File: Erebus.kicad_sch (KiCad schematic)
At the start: 1 part, among them U1 STM32F303CBTx

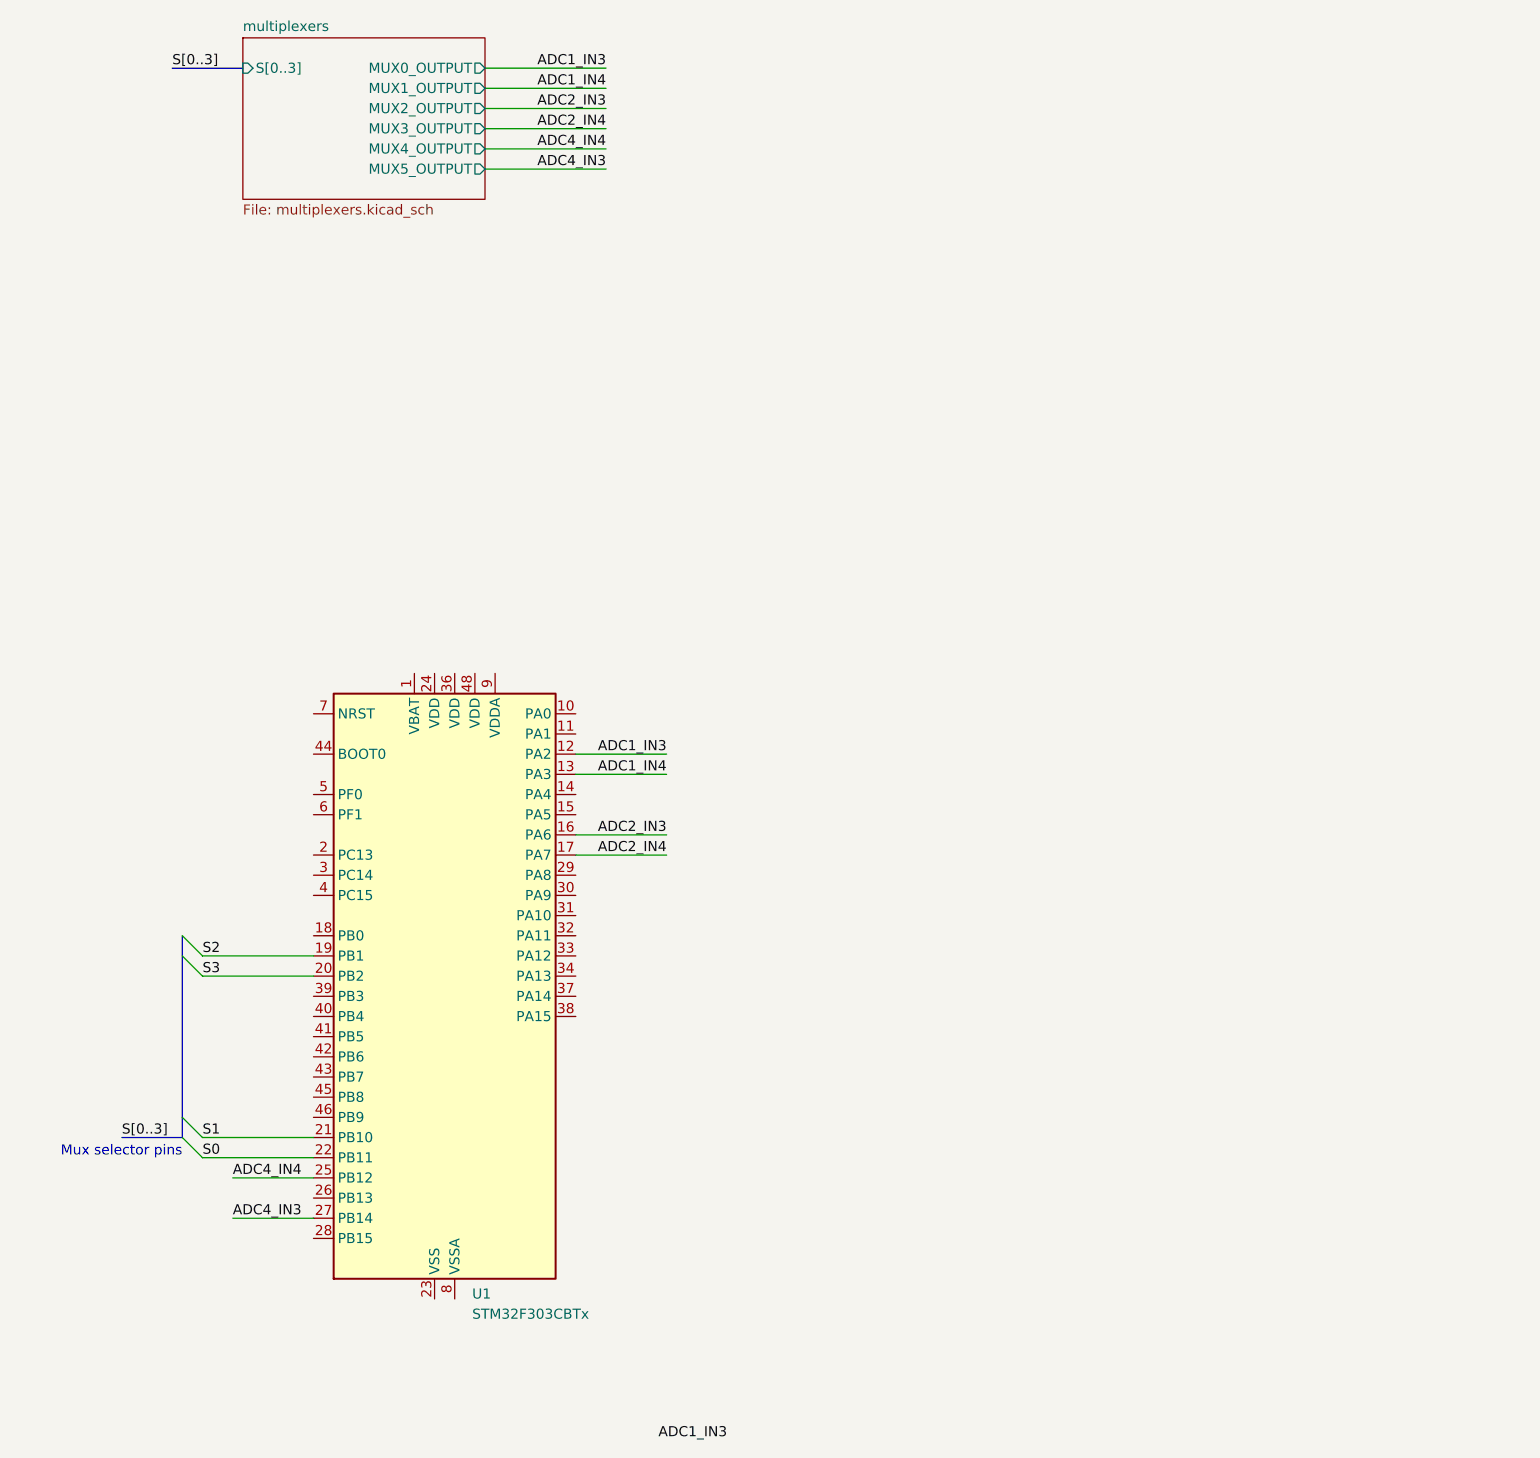
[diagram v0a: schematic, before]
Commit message: Setup Base Layout
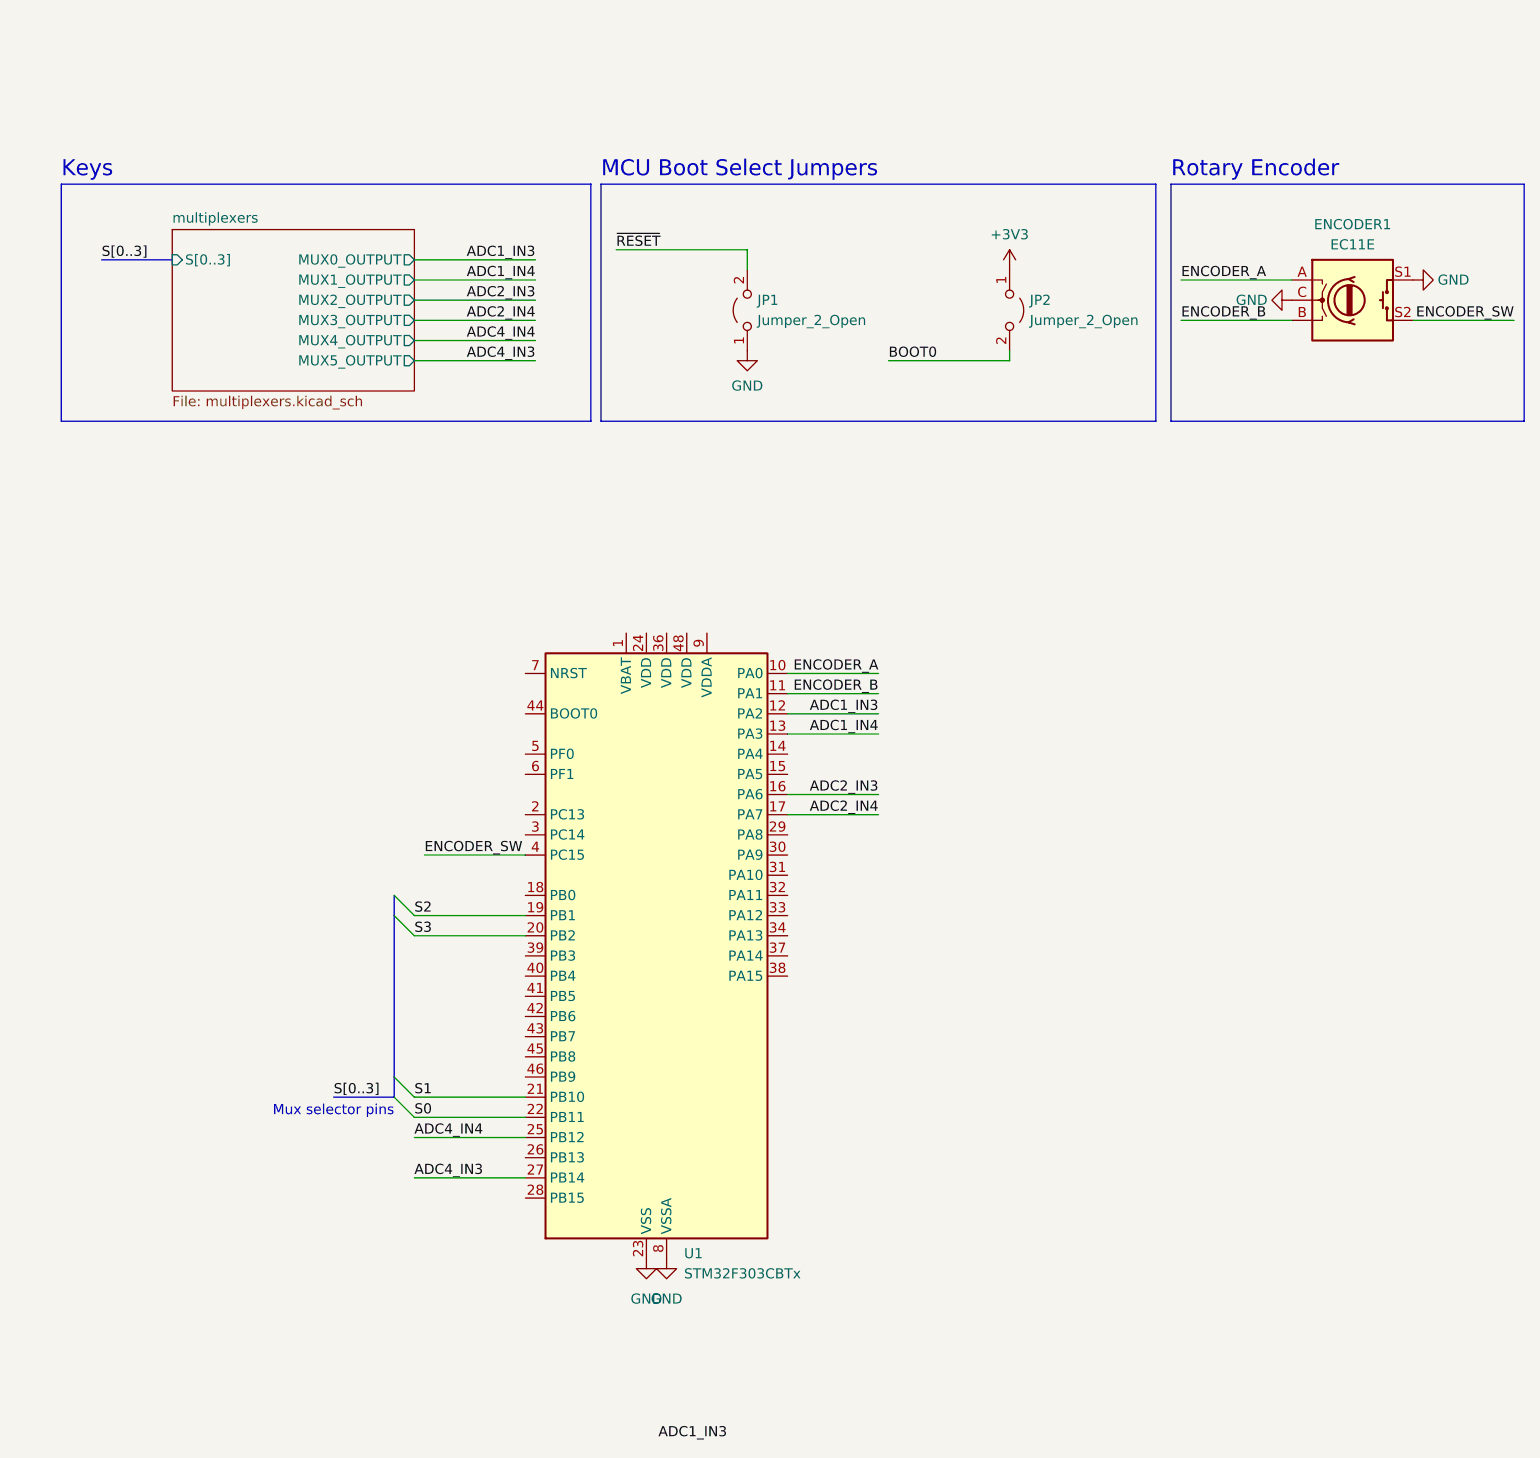
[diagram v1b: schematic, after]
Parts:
- added ENCODER1: EC11E, PCM_marbastlib-various:ROT_Alps_EC11E-Switch, symbol Device:RotaryEncoder_Switch
- added JP1, JP2: Jumper_2_Open, Connector_PinHeader_2.54mm:PinHeader_1x02_P2.54mm_Vertical, symbol Jumper:Jumper_2_Open
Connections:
- net ENCODER_A: now reaches U1.10 (PA0)
- net ENCODER_A: now also ENCODER1.A
- net ENCODER_B: now reaches U1.11 (PA1)
- net ENCODER_B: now also ENCODER1.B
- net GND: now reaches U1.23 (VSS), U1.35 (VSS), U1.47 (VSS)
- net GND: now also U1.8 (VSSA), ENCODER1.C, ENCODER1.S1, JP1.1 (A)
- net ENCODER_SW: now reaches U1.4 (PC15)
- net ENCODER_SW: now also ENCODER1.S2
- new net +3V3: JP2.1 (A)
- new net BOOT0: JP2.2 (B)
- new net ~{RESET}: JP1.2 (B)
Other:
- note added: "Keys"
- note added: "MCU Boot Select Jumpers"
- note added: "Rotary Encoder"
- moved on the sheet: U1
